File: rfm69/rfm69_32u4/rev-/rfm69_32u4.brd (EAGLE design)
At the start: 69.8 x 69.8 mm, 36 parts, among them K1 G5LE, SW1 SPST_TACT-KMR2, U1 433MHz, X2 USB-A, Y1 8MHz

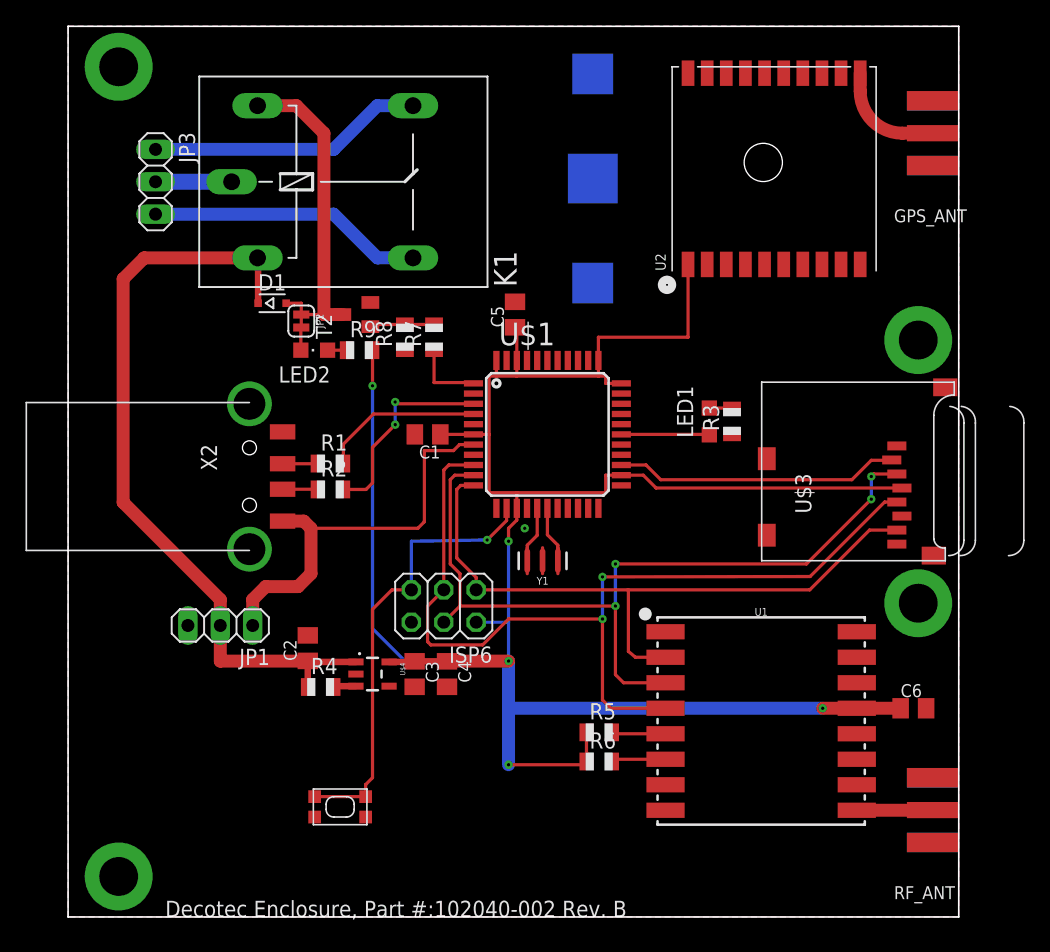
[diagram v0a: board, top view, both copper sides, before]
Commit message: minor changes
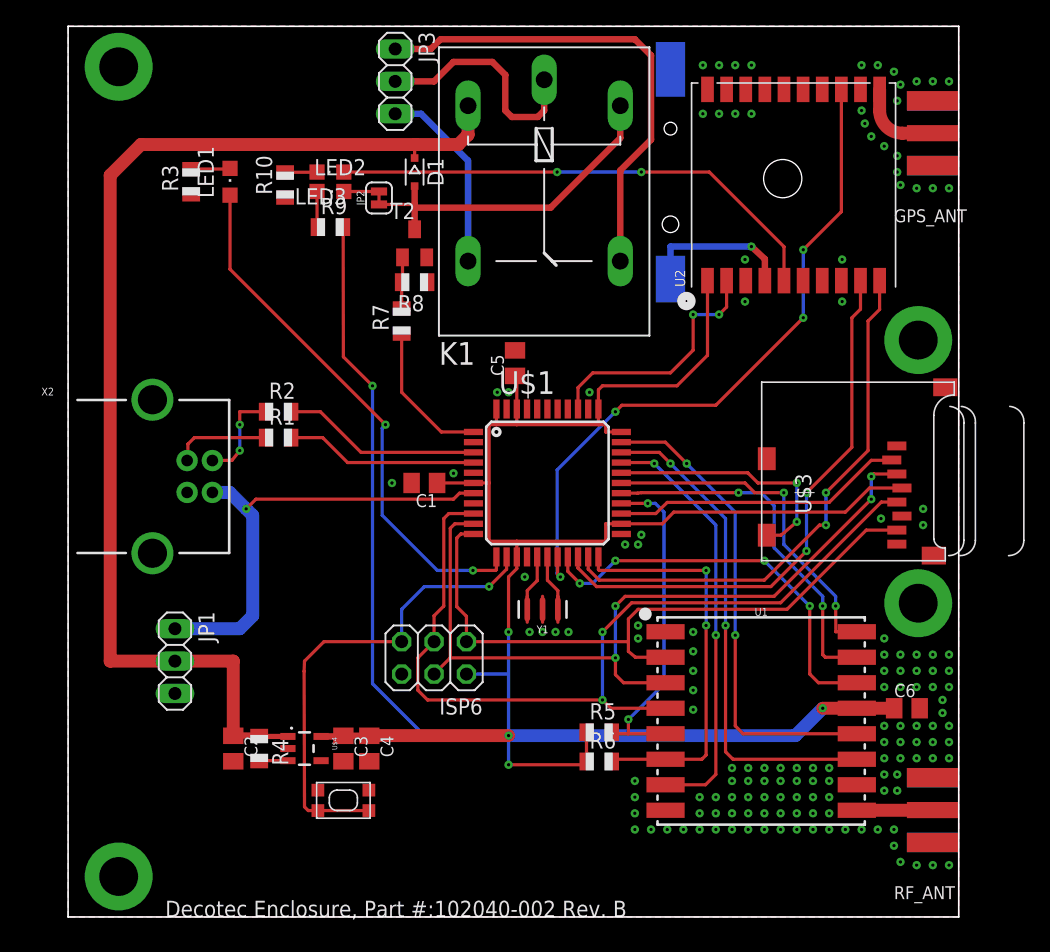
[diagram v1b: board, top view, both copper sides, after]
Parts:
- added LED3: FIX, adafruit:CHIPLED_0805
- added R10: 10k, adafruit:R0805
- LED2: value (none) -> RELAY
- U$5: value (none) -> CH291-1220LF; device adafruit:CR1220-SMD -> battery:CH291-1220LF
- X2: value USB-A -> USB_B_PTH; device adafruit:MOLEX_480371000 -> SparkFun-Connectors:USB-B-PTH
- moved R3 46.4 mm to (9.65, 57.7)
- moved LED1 42.0 mm to (12.7, 57.7)
- moved JP3 20.4 mm to (25.7, 65.5)
- moved D1 15.2 mm to (27.2, 58.4), turned to 270 degrees
- moved K1 15.1 mm to (37.3, 56.1), turned to 270 degrees
- moved LED2 12.5 mm to (20.6, 56.9), turned to 270 degrees
- moved JP2 11.4 mm to (24.4, 56.4), turned to 90 degrees
- moved R9 9.92 mm to (20.6, 54.1)
- moved C2 9.80 mm to (13.0, 13.2), turned to 270 degrees
- moved X2 8.89 mm to (5.33, 34.5), turned to 0 degrees
- moved C4 8.44 mm to (23.6, 13.2)
- moved U$5 8.27 mm to (47.2, 52.3), turned to 0 degrees
- moved C3 8.08 mm to (21.6, 13.2)
- moved U$4 7.91 mm to (18.5, 13.2)
- moved R2 7.33 mm to (16.5, 39.6)
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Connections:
- net A4_RF_RST renamed A4
- removed net 10: U$1.30
- removed net 11: U$1.12
- removed net 13: U$1.32
- removed net 5: U$1.31
- removed net 6: U$1.27
- removed net 8: LED1.A, U$1.28
- removed net A0: U$1.36
- removed net GPS_PPS: U$1.18
- removed net GPS_RST: U2.P$2
- removed net GPS_RXD: U2.P$10
- removed net GPS_TXD: U2.P$9
- removed net PPS: U2.P$13
- removed net RF_RST: R6.2, U1.6
- removed net TXLED: U$1.22
- removed net X_RF_DIO1: U1.15
- removed net X_RF_DIO2: U1.16
- removed net X_RF_DIO3: U1.11
- removed net X_RF_DIO4: U1.12
- removed net X_RF_DIO5: U1.7
- new net 10_RF_DIO5: U$1.30, U1.7
- new net 11_LED: LED1.A, U$1.12
- new net 13_RF_DIO4: U$1.32, U1.12
- new net 22_RF_RST: R6.2, U$1.22, U1.6
- new net 3_GPS_PPS: U$1.18, U2.P$13
- new net 5_RF_DIO3: U$1.31, U1.11
- new net 6_RF_DIO1: U$1.27, U1.15
- new net 8_RF_DIO2: U$1.28, U1.16
- new net A0_GPS_RST: U$1.36, U2.P$2
- new net N$5: LED3.C, R10.2
- net 0_GPS_TXD: now also U2.P$9
- net 1_GPS_RXD: now also U2.P$10
- net 3D-FIX: now also LED3.A
- net GND: now also R10.1, U$5.-, X2.GND; no longer X2.4
- net N$1: now also X2.D+; no longer X2.3
- net N$3: now also X2.D-; no longer X2.2
- net VBACKUP: now also U$5.+
- net VBUS: now also X2.VBUS; no longer X2.1
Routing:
- net 3_GPS_PPS: track 0.00 -> 53.5 mm, vias 0 -> 4
- net 0_GPS_TXD: track 0.00 -> 43.5 mm, vias 0 -> 2
- net 1_GPS_RXD: track 0.00 -> 42.7 mm, vias 0 -> 2
- net 11_LED: track 0.00 -> 42.0 mm, vias 0 -> 2
- net 3D-FIX: track 0.00 -> 39.6 mm, vias 0 -> 2
- net 5_RF_DIO3: track 0.00 -> 39.1 mm, vias 0 -> 2
- net 13_RF_DIO4: track 0.00 -> 37.8 mm, vias 0 -> 2
- net 10_RF_DIO5: track 0.00 -> 33.3 mm, vias 0 -> 2
- net 2_RF_DIO0: track 0.00 -> 32.0 mm, vias 0 -> 4
- net 22_RF_RST: track 0.00 -> 31.5 mm, vias 0 -> 2
- net VIN: track 60.7 -> 91.1 mm
- net 6_RF_DIO1: track 0.00 -> 28.4 mm, vias 0 -> 2
- net 8_RF_DIO2: track 0.00 -> 27.3 mm, vias 0 -> 2
- net 12_RF_CS: track 4.25 -> 26.4 mm, vias 0 -> 2
- net +3V3: track 185.2 -> 206.8 mm
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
